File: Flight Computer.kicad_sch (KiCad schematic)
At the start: 14 parts

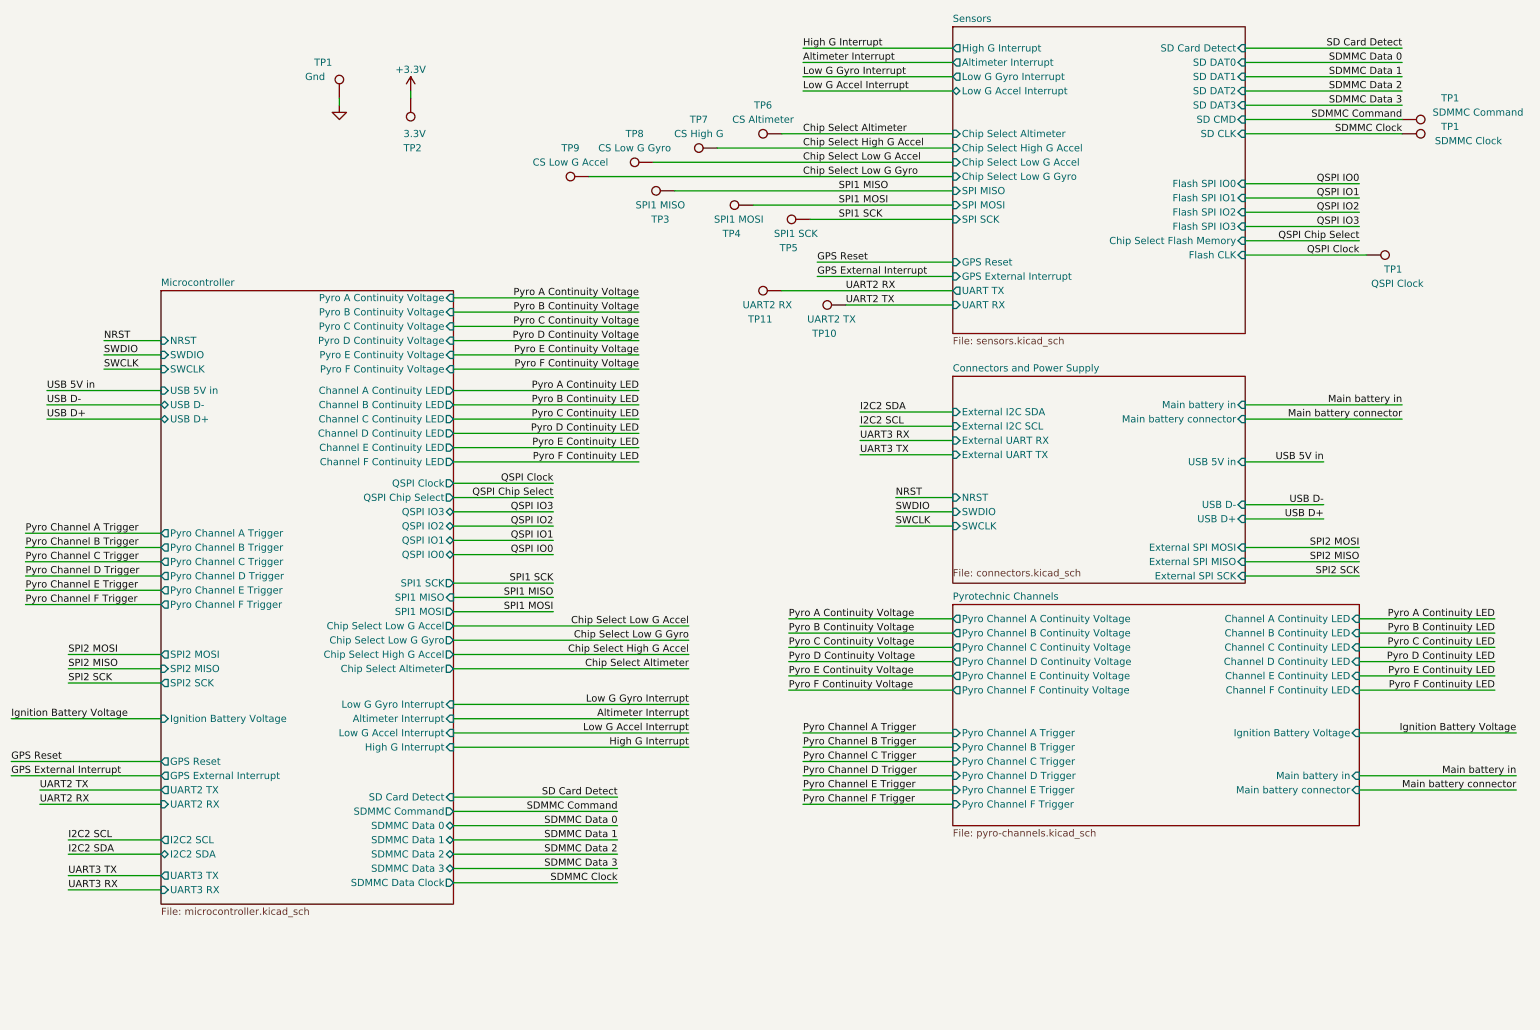
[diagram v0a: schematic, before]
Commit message: Swapped out sensors in schematic for v3
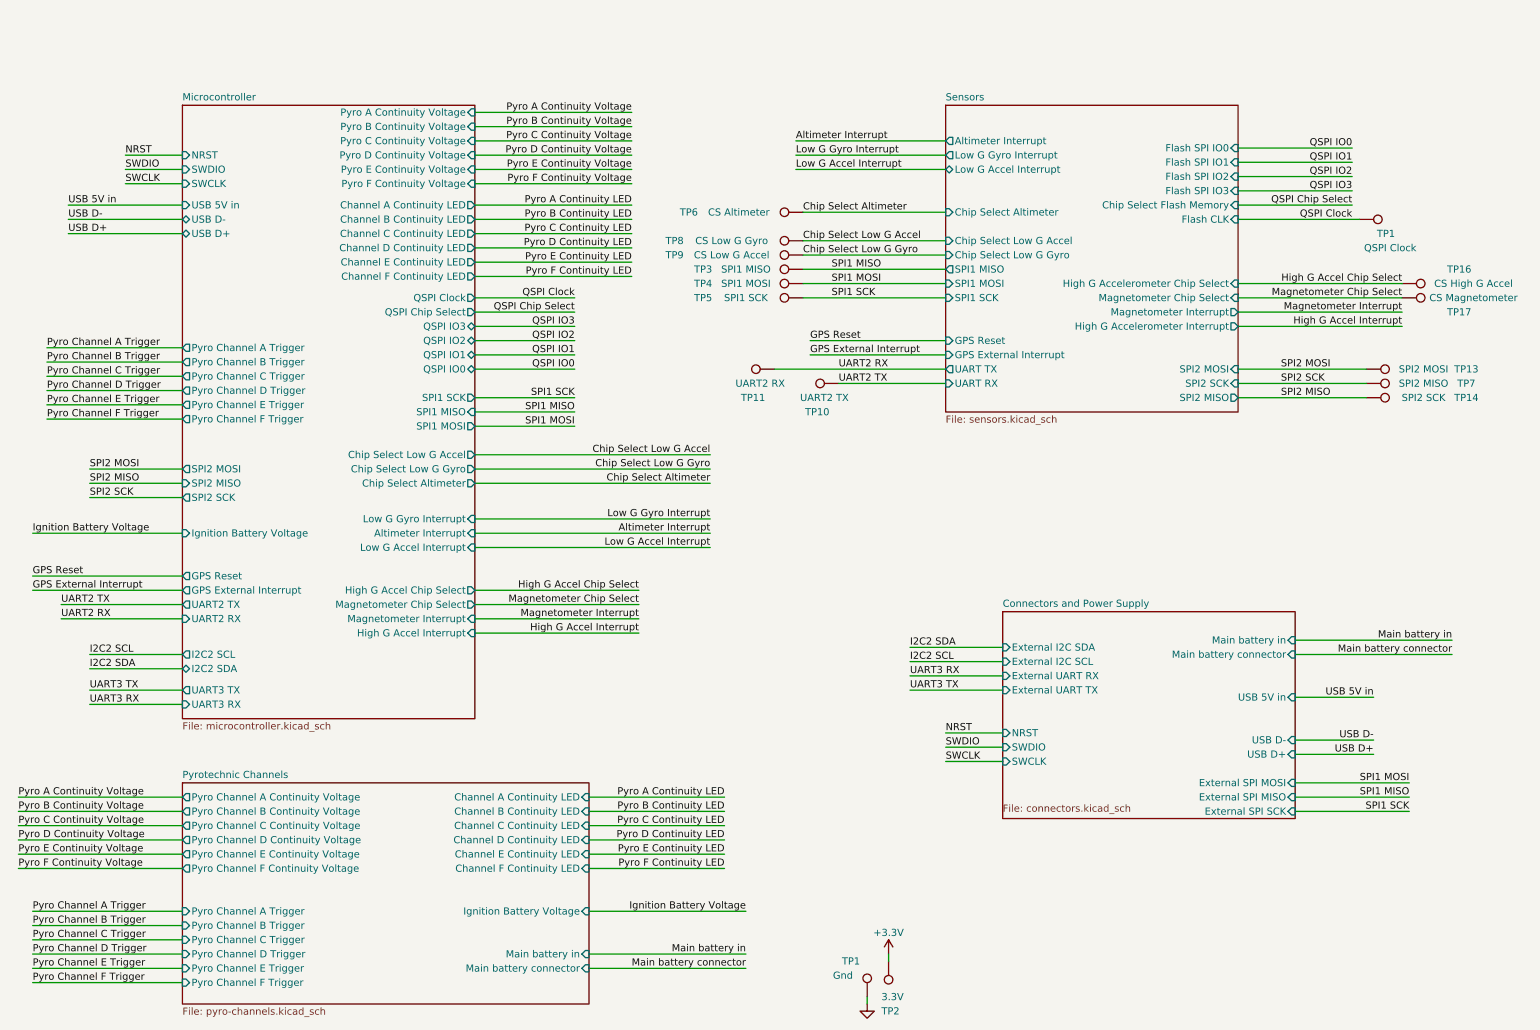
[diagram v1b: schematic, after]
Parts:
- removed TP1: SDMMC Clock, TestPoint:TestPoint_Pad_D1.5mm, symbol Connector:TestPoint
- removed TP1: SDMMC Command, TestPoint:TestPoint_Pad_D1.5mm, symbol Connector:TestPoint
- added TP13: SPI2 MOSI, TestPoint:TestPoint_Pad_D1.5mm, symbol Connector:TestPoint
- added TP14: SPI2 SCK, TestPoint:TestPoint_Pad_D1.5mm, symbol Connector:TestPoint
- added TP16: CS High G Accel, TestPoint:TestPoint_Pad_D1.5mm, symbol Connector:TestPoint
- added TP17: CS Magnetometer, TestPoint:TestPoint_Pad_D1.5mm, symbol Connector:TestPoint
- TP7: value CS High G -> SPI2 MISO
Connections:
- net Chip Select High G Accel is gone; now on net SPI2 SCK: TP7.1
- net SPI2 MISO: now also TP14.1
- net SPI2 MOSI: now also TP13.1
- new net High G Accel Chip Select: TP16.1
- new net Magnetometer Chip Select: TP17.1
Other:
- sheet Microcontroller ports: added High G Accel Chip Select, High G Accel Interrupt, Magnetometer Chip Select, Magnetometer Interrupt; removed Chip Select High G Accel, High G Interrupt, SD Card Detect, SDMMC Command, SDMMC Data 0, SDMMC Data 1, SDMMC Data 2, SDMMC Data 3, SDMMC Data Clock
- sheet Sensors ports: added High G Accelerometer Chip Select, High G Accelerometer Interrupt, Magnetometer Chip Select, Magnetometer Interrupt, SPI1 MISO, SPI1 MOSI, SPI1 SCK, SPI2 MISO, SPI2 MOSI, SPI2 SCK; removed Chip Select High G Accel, High G Interrupt, SD CLK, SD CMD, SD Card Detect, SD DAT0, SD DAT1, SD DAT2, SD DAT3, SPI MISO, SPI MOSI, SPI SCK
- moved on the sheet: TP1, TP10, TP11, TP2, TP3, TP4, TP5, TP6, TP8, TP9
